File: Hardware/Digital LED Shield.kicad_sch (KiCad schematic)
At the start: 13 parts, among them J1 Conn_02x10_Odd_Even, J2 Conn_01x03_Male, J3 Barrel_Jack_MountingPin, J4 Conn_01x02_Female, U1 SN74LVC1T45DBV

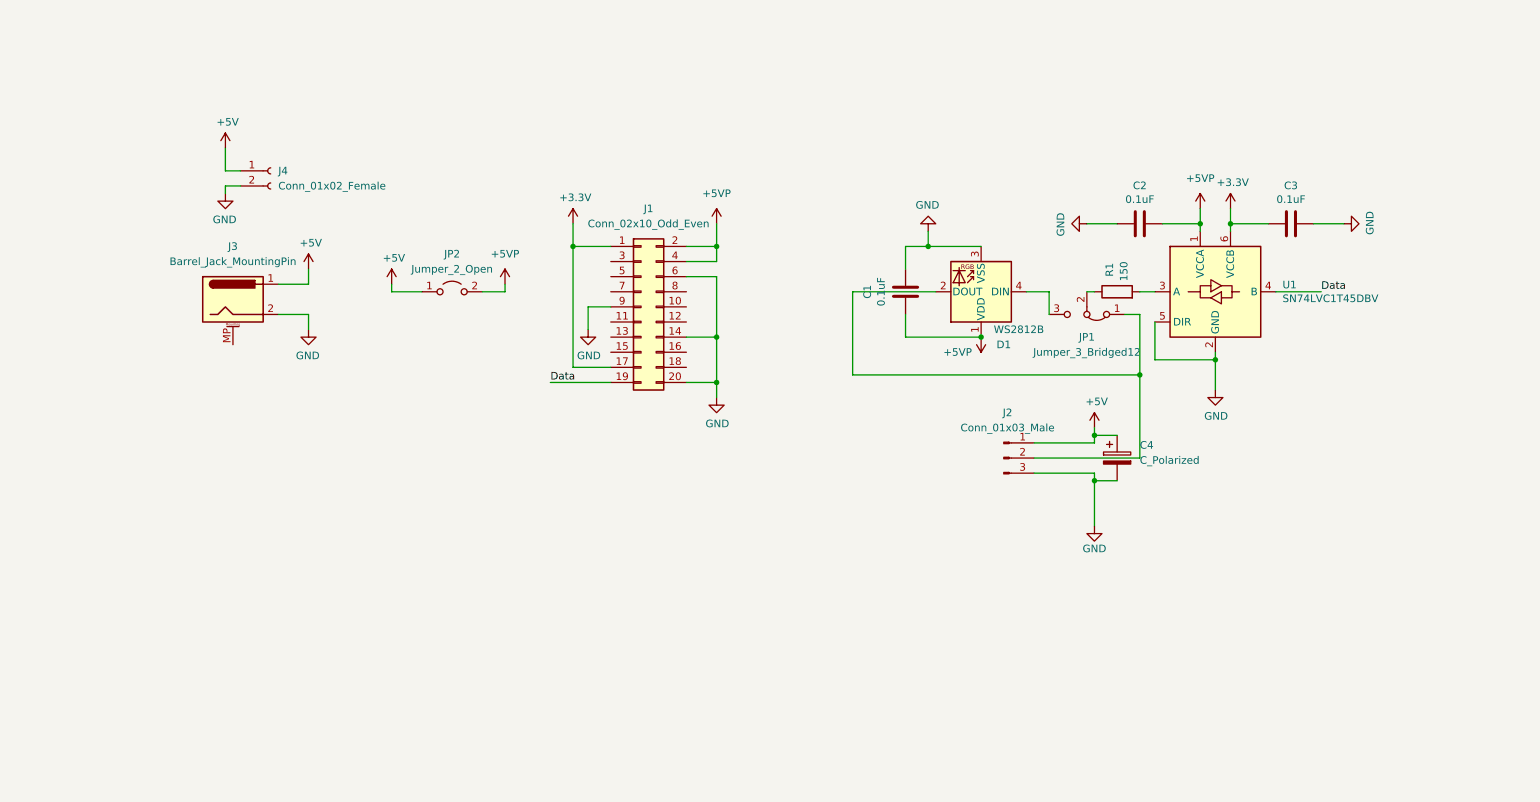
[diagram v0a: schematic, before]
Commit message: add protection
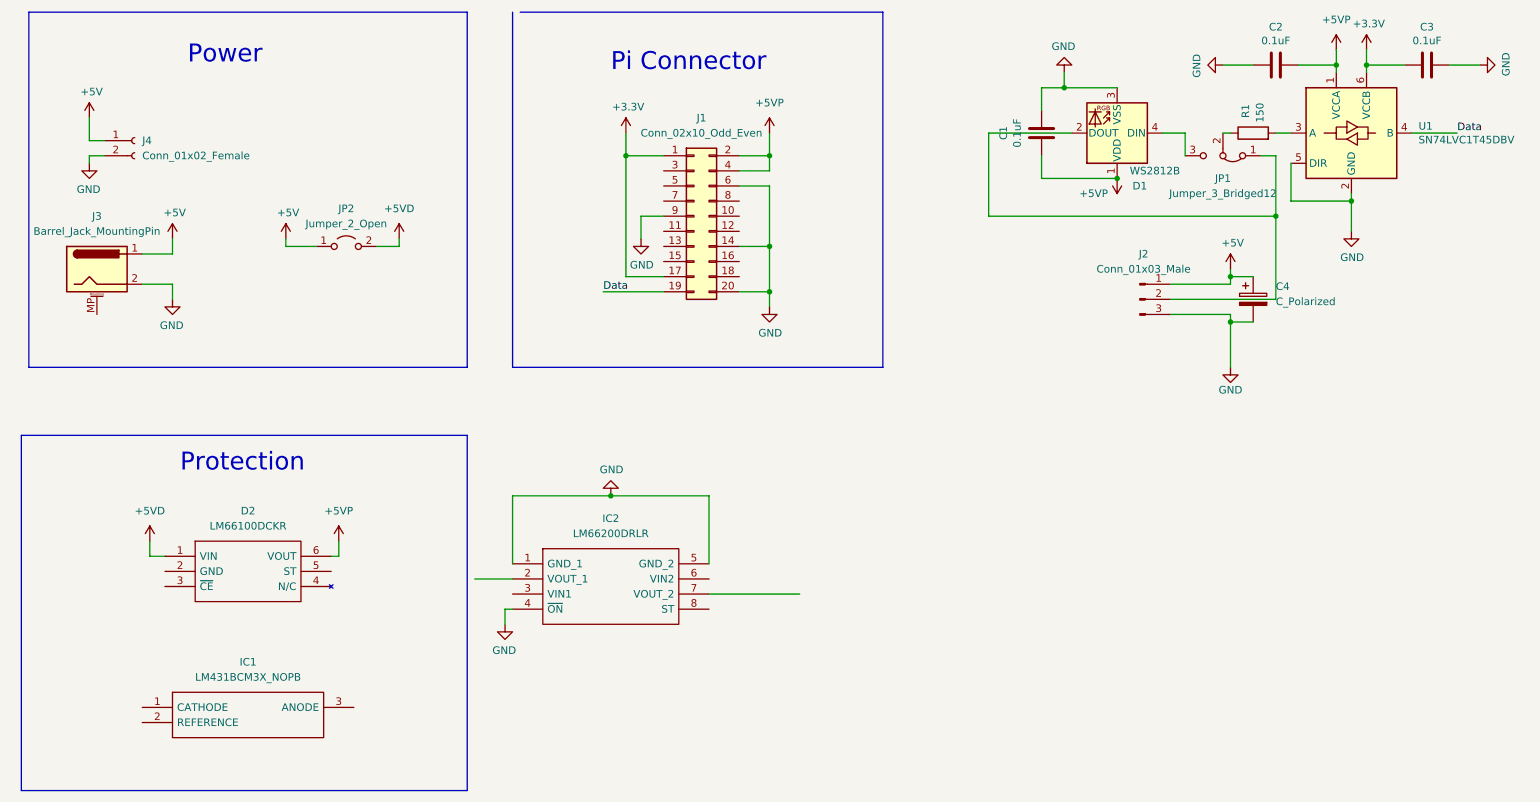
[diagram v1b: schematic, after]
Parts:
- added D2: LM66100DCKR, SOP65P210X110-6N, symbol LM66100DCKR:LM66100DCKR
- added IC1: LM431BCM3X_NOPB, LM431BCM3X:SOT95P237X95-3N, symbol LM431BCM3X_NOPB:LM431BCM3X_NOPB
- added IC2: LM66200DRLR, SOTFL50P160X60-8N, symbol LM66200DRLR:LM66200DRLR
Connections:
- net +5VP: now also D2.6 (VOUT); no longer JP2.2 (B)
- net GND: now also IC2.1 (GND_1), IC2.4 (~{ON}), IC2.5 (GND_2)
- new net +5VD: D2.1 (VIN), JP2.2 (B)
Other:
- note added: "Pi Connector"
- note added: "Power"
- note added: "Protection"
- moved on the sheet: C1, C2, C3, C4, D1, J1, J2, J3, J4, JP1, JP2, R1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
